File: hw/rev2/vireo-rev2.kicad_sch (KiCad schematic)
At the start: 0 parts

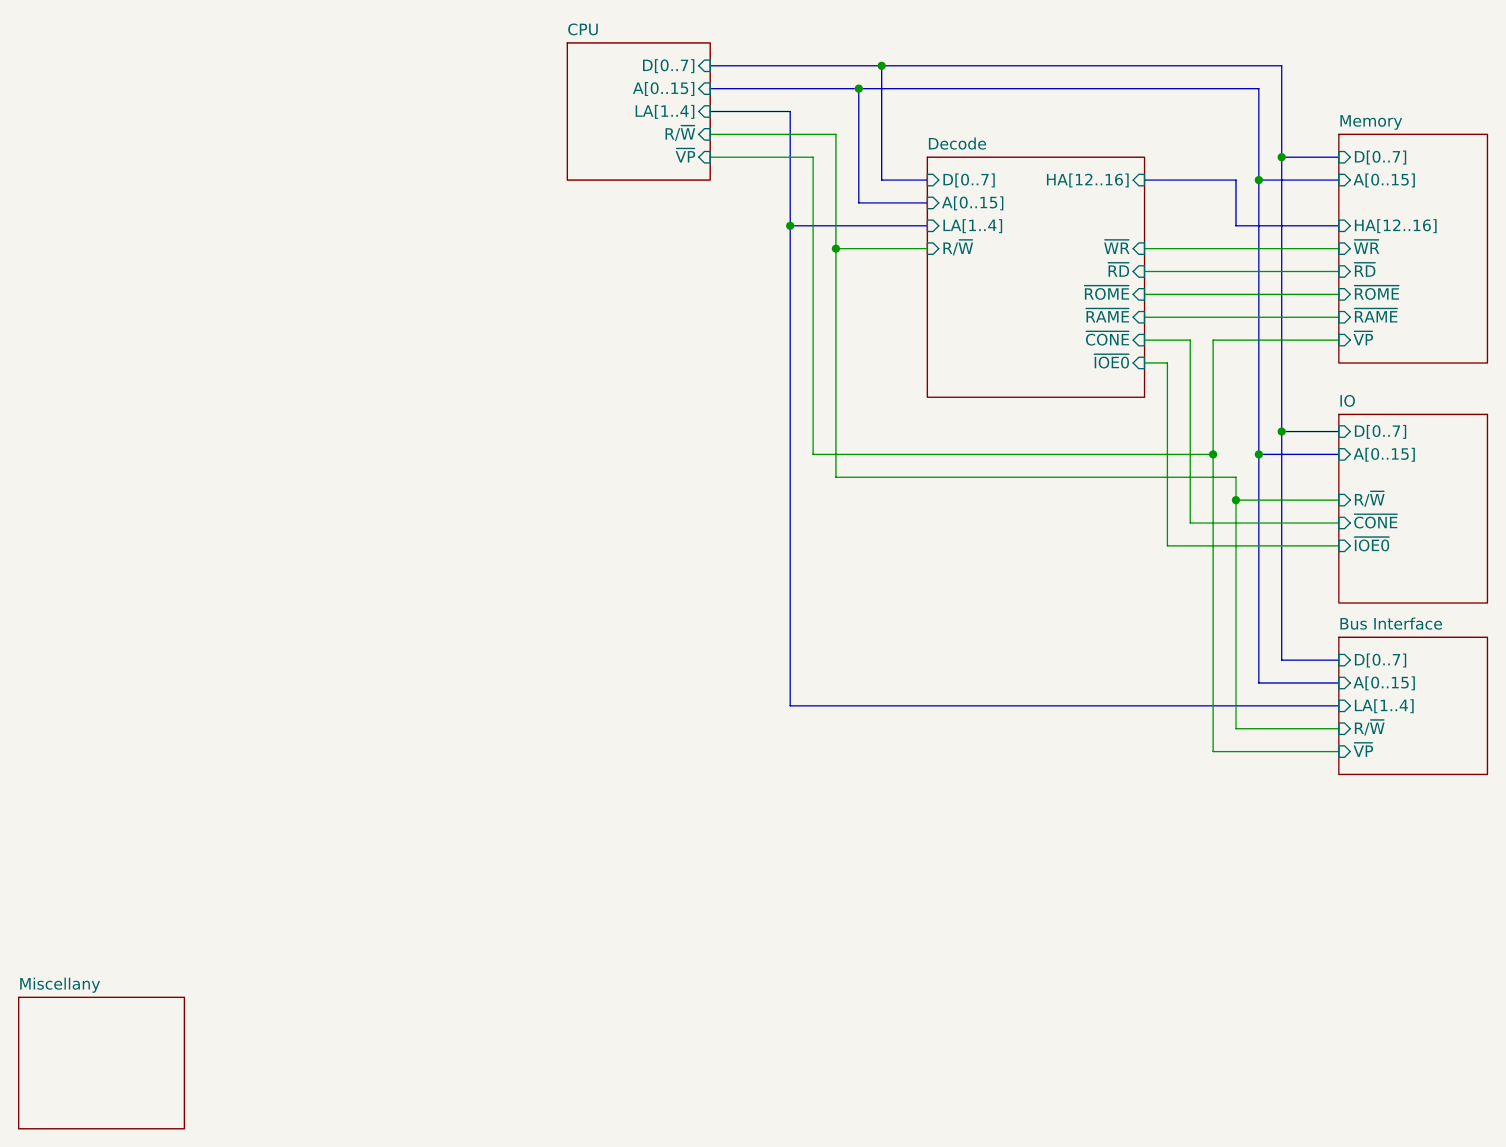
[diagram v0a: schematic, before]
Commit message: hardware revisions
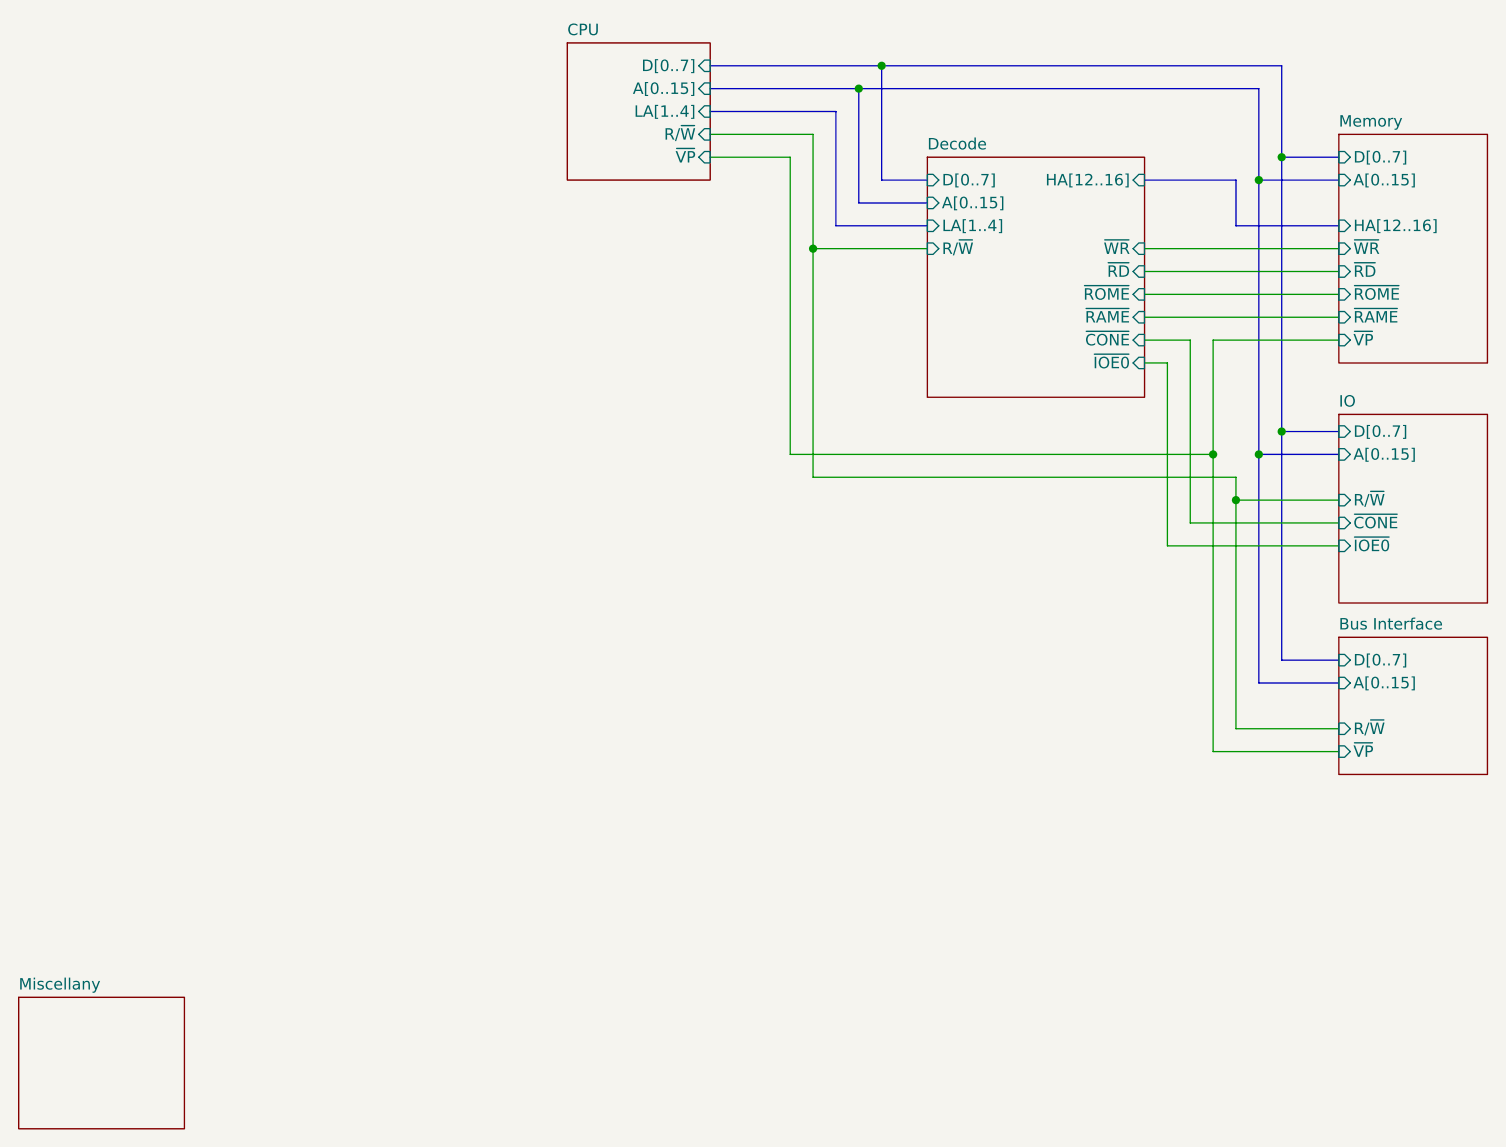
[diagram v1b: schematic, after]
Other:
- sheet Bus Interface ports: added none; removed LA[1..4]
- title: (none) -> Vireo Microcomputer
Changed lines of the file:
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@@
 	(generator_version "9.0")
 	(paper "USLetter")
+	(title_block
+		(title "Vireo Microcomputer")
+		(date "2025-07-27")
+		(rev "2")
+	)
 	(junction
 		(at 156.21 110.49)
@@
 	)
 	(junction
-		(at 109.22 85.09)
+		(at 111.76 87.63)
 		(diameter 0)
 		(color 0 0 0 0)
@@
 		(color 0 0 0 0)
 	)
-	(junction
-		(at 114.3 87.63)
-		(diameter 0)
-		(color 0 0 0 0)
-	)
 	(wire
 		(pts
@@
 	(wire
 		(pts
-			(xy 114.3 74.93) (xy 114.3 87.63)
+			(xy 111.76 74.93) (xy 111.76 87.63)
 		)
 		(stroke
@@
 		)
 	)
-	(wire
-		(pts
-			(xy 114.3 87.63) (xy 114.3 113.03)
-		)
-		(stroke
-			(width 0)
-			(type default)
-		)
-	)
-	(bus
-		(pts
-			(xy 109.22 72.39) (xy 109.22 85.09)
-		)
-		(stroke
-			(width 0)
-			(type default)
-		)
-	)
 	(bus
 		(pts
@@
 	(wire
 		(pts
-			(xy 111.76 110.49) (xy 156.21 110.49)
+			(xy 109.22 110.49) (xy 156.21 110.49)
 		)
 		(stroke
@@
 	(wire
 		(pts
-			(xy 114.3 113.03) (xy 158.75 113.03)
+			(xy 111.76 113.03) (xy 158.75 113.03)
 		)
 		(stroke
@@
 	(bus
 		(pts
-			(xy 109.22 85.09) (xy 124.46 85.09)
-		)
-		(stroke
-			(width 0)
-			(type default)
-		)
-	)
-	(bus
-		(pts
 			(xy 119.38 67.31) (xy 119.38 80.01)
 		)
@@
 	(wire
 		(pts
-			(xy 114.3 87.63) (xy 124.46 87.63)
-		)
-		(stroke
-			(width 0)
-			(type default)
-		)
-	)
-	(wire
-		(pts
 			(xy 148.59 90.17) (xy 170.18 90.17)
 		)
@@
 	(wire
 		(pts
-			(xy 111.76 77.47) (xy 111.76 110.49)
+			(xy 109.22 77.47) (xy 109.22 110.49)
 		)
 		(stroke
@@
 	(wire
 		(pts
-			(xy 100.33 77.47) (xy 111.76 77.47)
+			(xy 100.33 77.47) (xy 109.22 77.47)
 		)
 		(stroke
@@
 	(bus
 		(pts
-			(xy 109.22 138.43) (xy 170.18 138.43)
-		)
-		(stroke
-			(width 0)
-			(type default)
-		)
-	)
-	(bus
-		(pts
 			(xy 148.59 80.01) (xy 158.75 80.01)
 		)
@@
 	(bus
 		(pts
+			(xy 100.33 72.39) (xy 114.3 72.39)
+		)
+		(stroke
+			(width 0)
+			(type default)
+		)
+	)
+	(bus
+		(pts
 			(xy 161.29 69.85) (xy 161.29 80.01)
 		)
@@
 	(wire
 		(pts
-			(xy 100.33 74.93) (xy 114.3 74.93)
+			(xy 100.33 74.93) (xy 111.76 74.93)
 		)
 		(stroke
@@
 		)
 	)
+	(bus
+		(pts
+			(xy 114.3 72.39) (xy 114.3 85.09)
+		)
+		(stroke
+			(width 0)
+			(type default)
+		)
+	)
 	(wire
 		(pts
@@
 	(wire
 		(pts
+			(xy 111.76 87.63) (xy 124.46 87.63)
+		)
+		(stroke
+			(width 0)
+			(type default)
+		)
+	)
+	(bus
+		(pts
+			(xy 114.3 85.09) (xy 124.46 85.09)
+		)
+		(stroke
+			(width 0)
+			(type default)
+		)
+	)
+	(wire
+		(pts
 			(xy 148.59 92.71) (xy 170.18 92.71)
 		)
@@
 		)
 	)
-	(bus
-		(pts
-			(xy 109.22 85.09) (xy 109.22 138.43)
+	(wire
+		(pts
+			(xy 111.76 87.63) (xy 111.76 113.03)
 		)
 		(stroke
@@
 		(pts
 			(xy 158.75 85.09) (xy 170.18 85.09)
-		)
-		(stroke
-			(width 0)
-			(type default)
-		)
-	)
-	(bus
-		(pts
-			(xy 100.33 72.39) (xy 109.22 72.39)
 		)
 		(stroke
@@
 		)
 		(instances
-			(project "sb6502-mk2"
+			(project "vireo-rev2"
 				(path "/8c8f1a65-1f54-40f3-b06e-5c7999916e29"
 					(page "2")
@@
 		)
 		(instances
-			(project "sb6502-mk2"
+			(project "vireo-rev2"
 				(path "/8c8f1a65-1f54-40f3-b06e-5c7999916e29"
 					(page "5")
@@
 		)
 		(instances
-			(project "sb6502-mk2"
+			(project "vireo-rev2"
 				(path "/8c8f1a65-1f54-40f3-b06e-5c7999916e29"
 					(page "7")
@@
 		)
 		(instances
-			(project "sb6502-mk2"
+			(project "vireo-rev2"
 				(path "/8c8f1a65-1f54-40f3-b06e-5c7999916e29"
 					(page "4")
@@
 		)
 		(instances
-			(project "sb6502-mk2"
+			(project "vireo-rev2"
 				(path "/8c8f1a65-1f54-40f3-b06e-5c7999916e29"
 					(page "3")
@@
 			)
 		)
-		(pin "LA[1..4]" input
-			(at 170.18 138.43 180)
-			(effects
-				(font
-					(size 1.27 1.27)
-				)
-				(justify left)
-			)
-		)
 		(instances
-			(project "sb6502-mk2"
+			(project "vireo-rev2"
 				(path "/8c8f1a65-1f54-40f3-b06e-5c7999916e29"
 					(page "6")
